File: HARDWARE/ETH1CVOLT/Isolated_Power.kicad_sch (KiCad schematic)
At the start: 91 parts, among them U15 RP-2424D, U16 TMR4-2423WI, U17 TEC2-2419WI, U18 TSR0.5-2465, U19 TPS7A3901DSCR, U20 TPS7A3901DSCR, U21 TPS7A3901DSCR, U22 ADP7142ARDZ-5.0, U23 ADP7142ARDZ-5.0

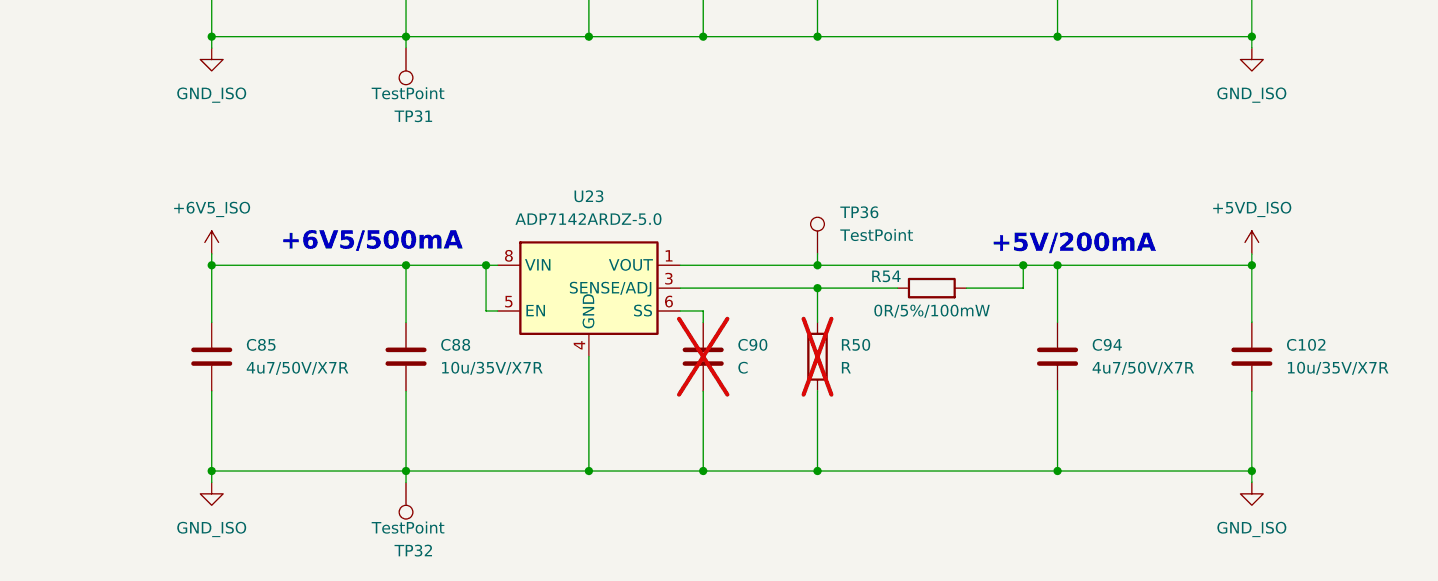
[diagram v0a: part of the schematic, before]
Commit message: Modifications
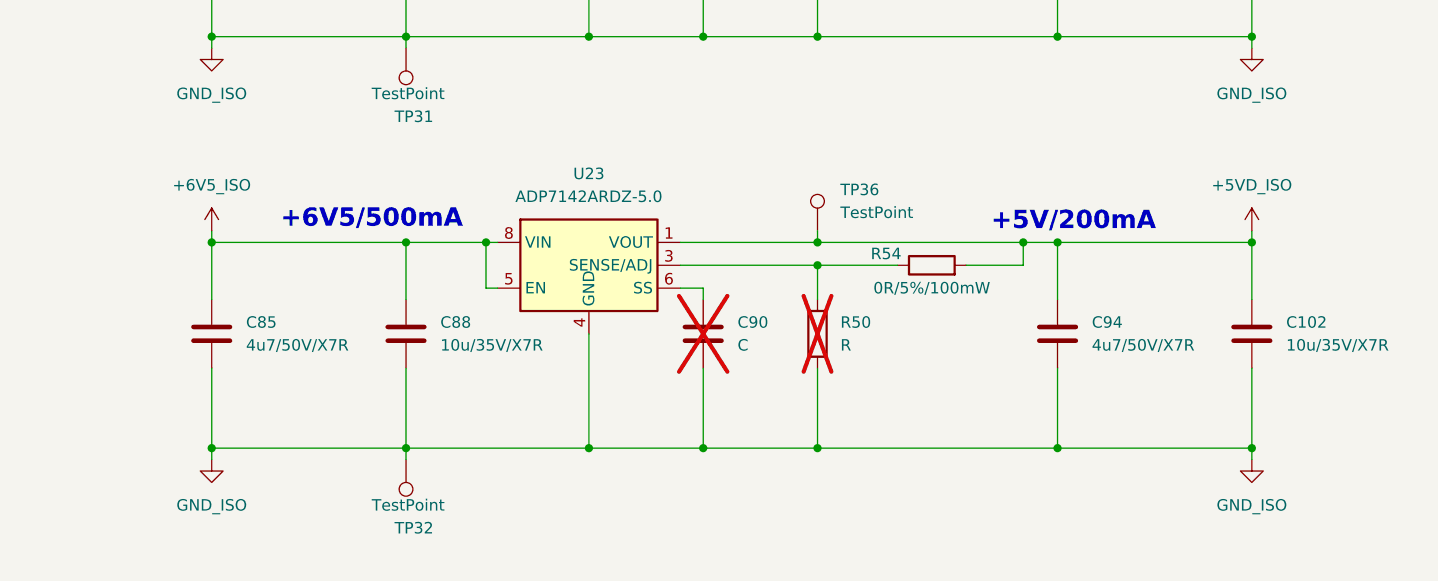
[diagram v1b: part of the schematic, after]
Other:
- moved on the sheet: C102, C85, C88, C90, C94, R50, R54, TP32, TP36, U23
